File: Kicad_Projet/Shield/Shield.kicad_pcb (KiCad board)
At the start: 2 copper layers, 68.6 x 53.3 mm, 25 parts, among them J1 Power, J2 Digital/PWM, J3 Analog, J4 Digital/PWM, U2 LTC1050

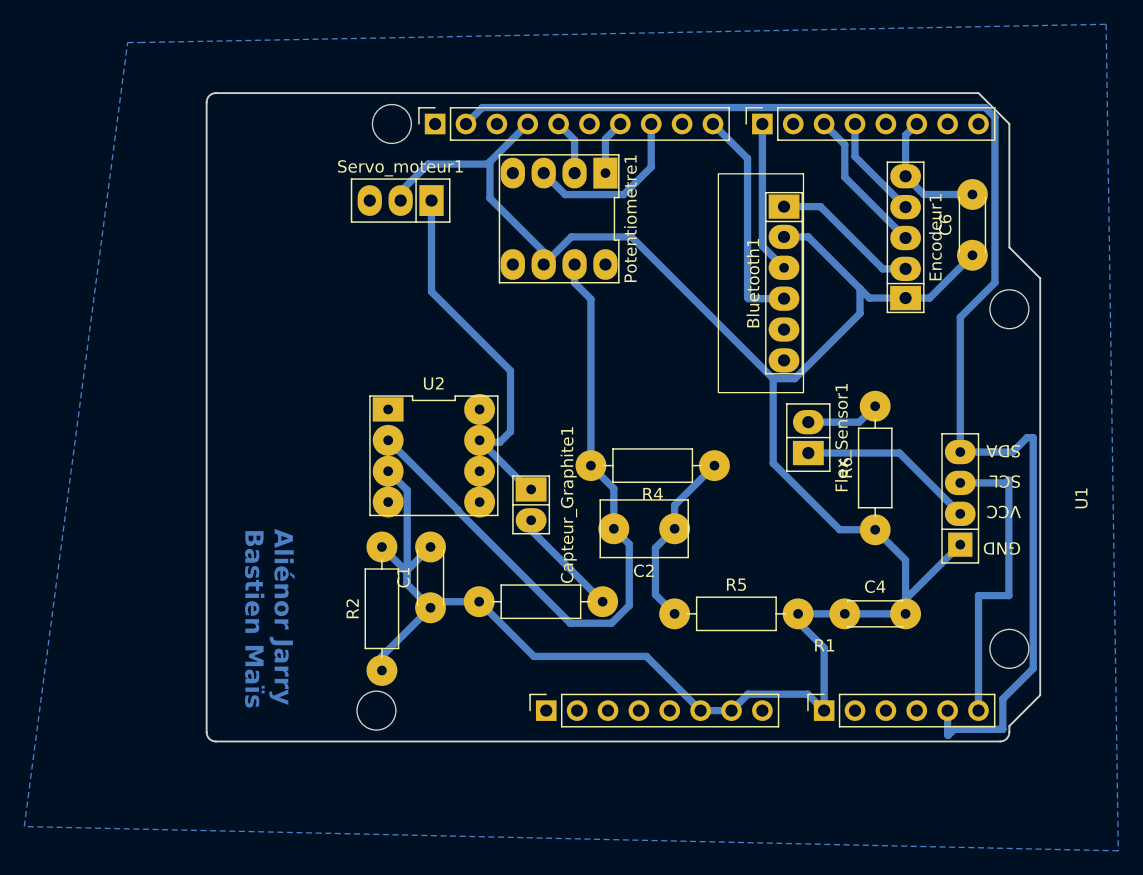
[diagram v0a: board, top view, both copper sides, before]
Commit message: pcb and mask
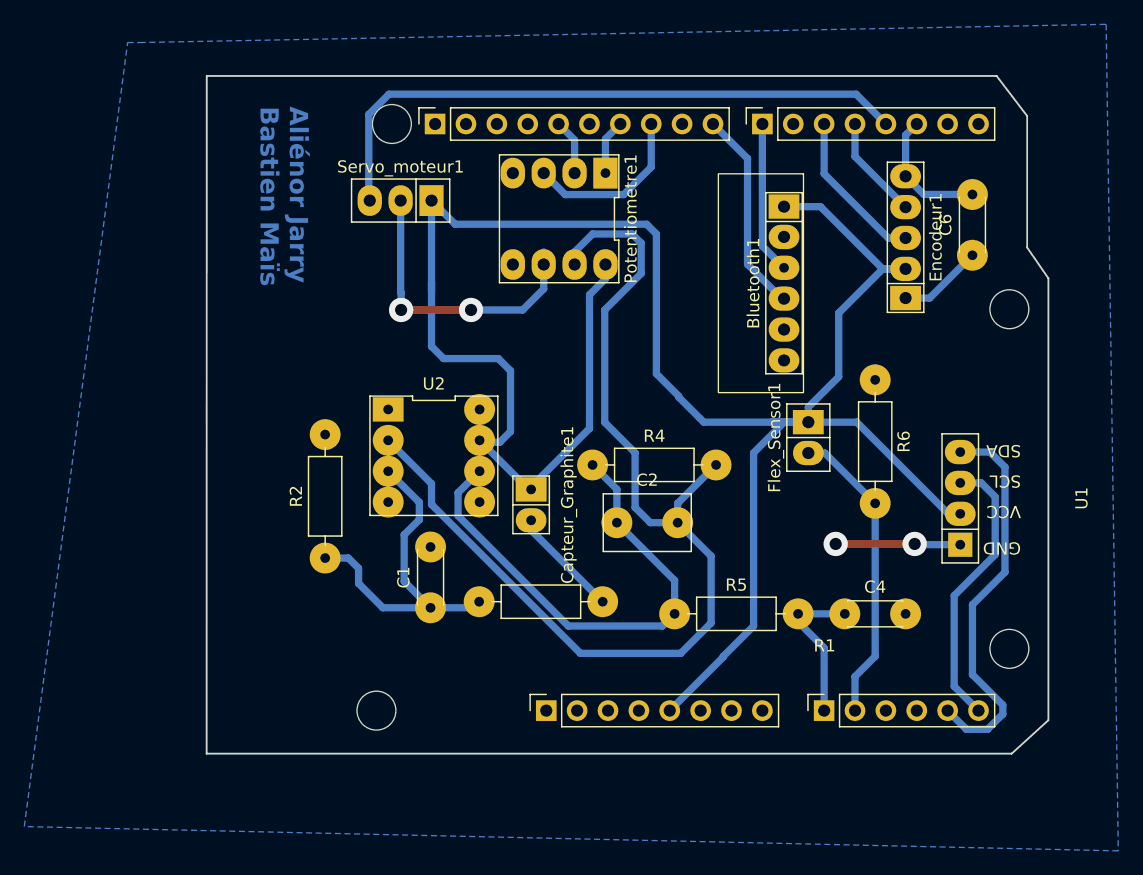
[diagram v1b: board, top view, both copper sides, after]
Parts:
- moved R6 12.3 mm to (155.0, 70.2), turned to -90 degrees
- moved R2 10.4 mm to (109.8, 84.9)
- moved R4 10.0 mm to (131.8, 77.2), turned to 0 degrees
- moved C2 4.78 mm to (133.8, 82.0), turned to 0 degrees
- turned Flex_Sensor1 to -90 degrees
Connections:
- net A4 renamed SDA
- Bluetooth1 pad 2: ADC -> GND
- C1 pad 1: ADC -> Net-(U2-+)
- C1 pad 2: ADC -> GND
- C4 pad 2: ADC -> GND
- C6 pad 1: ADC -> GND
- Encodeur1 pad 1: ADC -> GND
- J1 pad 6: ADC -> GND
- J1 pad 7: ADC -> GND
- J2 pad 4: ADC -> GND
- Potentiometre1 pad 4: unconnected-(Potentiometre1-VSS-Pad4) -> GND
- Potentiometre1 pad 6: ADC -> GND
- Potentiometre1 pad 8: unconnected-(Potentiometre1-VDD-Pad8) -> +5V
- R1 pad 2: ADC -> Net-(U2-+)
- R2 pad 1: ADC -> Net-(U2-+)
- R2 pad 2: ADC -> GND
- R6 pad 1: ADC -> GND
- Servo_moteur1 pad 2: ADC -> GND
- U1 pad 1: ADC -> GND
- U2 pad 3: ADC -> Net-(U2-+)
- U2 pad 4: ADC -> GND
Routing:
- net ADC: track 194.5 -> 13.9 mm
- net +5V: track 57.7 -> 175.9 mm
- net SDA: track 111.4 -> 32.4 mm
- net D3: track 0.00 -> 51.4 mm
- net GND: track 0.00 -> 43.5 mm, vias 0 -> 4
- net Net-(U2-+): track 0.00 -> 30.1 mm
- net R3: track 56.8 -> 86.8 mm
- net Net-(C2-Pad1): track 14.9 -> 41.6 mm
- net A1: track 6.04 -> 25.0 mm
- net SCL: track 25.8 -> 23.4 mm
- net RXD: track 18.5 -> 16.9 mm
- net SW: track 12.2 -> 13.0 mm
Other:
- board size 68.6 x 53.3 mm -> 69.2 x 55.8 mm
